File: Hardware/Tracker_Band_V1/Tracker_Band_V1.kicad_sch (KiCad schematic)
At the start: 78 parts, among them J1 USB_C_USB20, Q1 SSM6L56FE, SW1 EVP-AVAA1A, SW2 EVP-AVAA1A, U1 ESP32-C3-MINI-1-N4, U2 BNO085, U3 RT8010, U4 MCP73832-2-AC, U5 LM66200, U6 IN-PI15TAT5R5G5B, U7 IN-PI15TAT5R5G5B, U8 IN-PI15TAT5R5G5B, U9 IN-PI15TAT5R5G5B, X1 32.768kHz

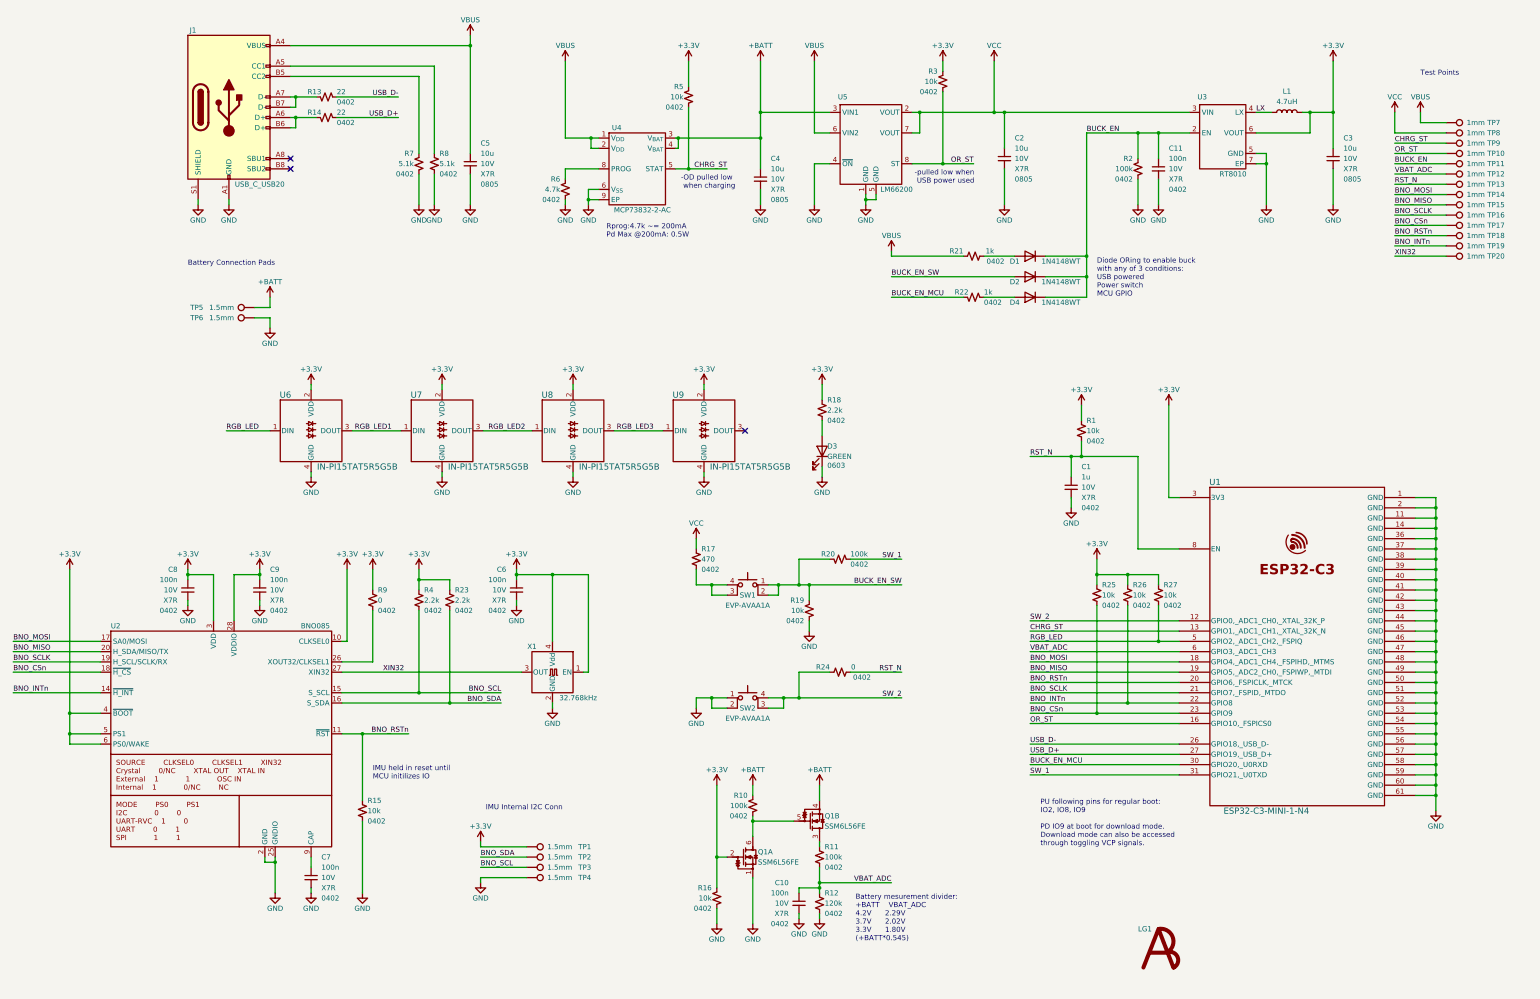
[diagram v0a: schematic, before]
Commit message: SCH & PCB Finalized for review
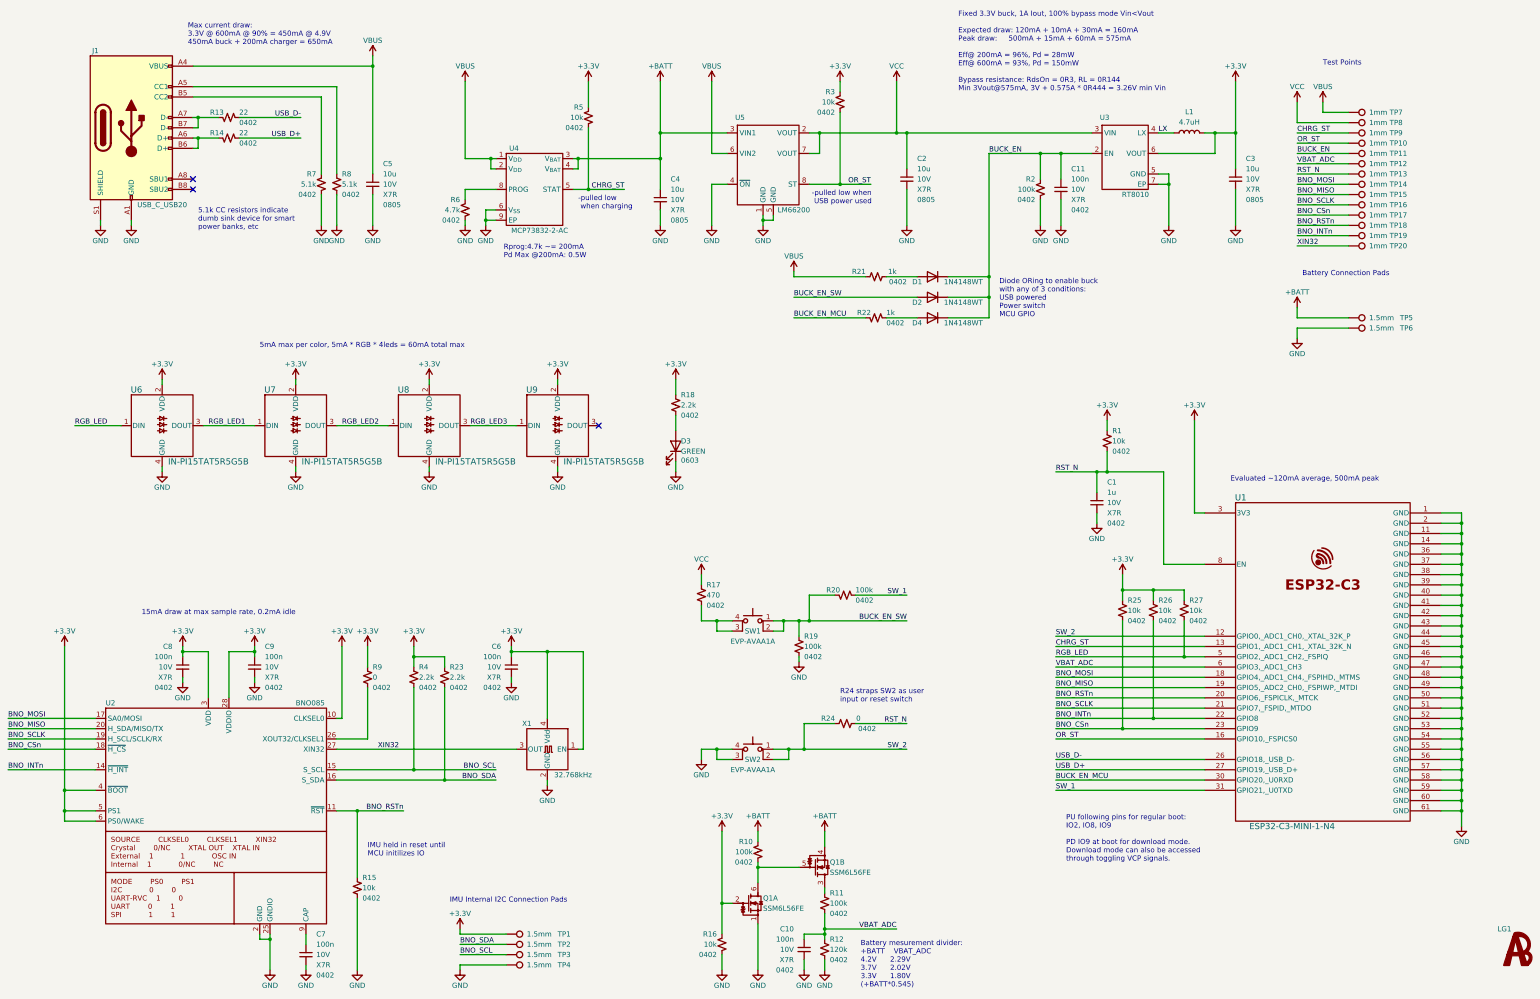
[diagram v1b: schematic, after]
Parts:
- R19: value 10k -> 100k
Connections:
- net GND: now also SW2.3 (K), SW2.4 (A); no longer SW2.1, SW2.2
- net SW_2: now also SW2.1, SW2.2; no longer SW2.3 (K), SW2.4 (A)
- now unconnected: U1.10 (NC), U1.15 (NC), U1.17 (NC), U1.24 (NC), U1.25 (NC), U1.28 (NC), U1.29 (NC), U1.32 (NC), U1.33 (NC), U1.34 (NC), U1.35 (NC), U1.4 (NC), U1.7 (NC), U1.9 (NC), U2.1 (PIN1), U2.12 (PIN12), U2.13 (PIN13), U2.21 (PIN21), U2.22 (PIN22), U2.23 (PIN23), U2.24 (PIN24), U2.7 (PIN7), U2.8 (PIN8)
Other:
- note added: "-pulled low when charging"
- note added: "15mA draw at max sample rate, 0.2mA idle"
- note added: "5.1k CC resistors indicate dumb sink device for smart power banks, etc"
- note added: "5mA max per color, 5mA * RGB * 4leds = 60mA total max"
- note added: "Evaluated ~120mA average, 500mA peak"
- note added: "Fixed 3.3V buck, 1A Iout, 100% bypass mode Vin<Vout Expected draw: 120mA + 10mA + 30mA = 160mA Peak draw: 500mA + 15mA + 60mA = 575mA Eff@ 200mA = 96%, Pd = 28mW Eff@ 600mA = 93%, Pd = 150mW Bypass resistance: RdsOn = 0R3, RL = 0R144 Min 3Vout@575mA, 3V + 0.575A * 0R444 = 3.26V min Vin"
- note added: "IMU Internal I2C Connection Pads"
- note added: "Max current draw: 3.3V @ 600mA @ 90% = 450mA @ 4.9V 450mA buck + 200mA charger = 650mA"
- note added: "R24 straps SW2 as user input or reset switch"
- note removed: "-OD pulled low when charging"
- note removed: "IMU Internal I2C Conn"
- company: (none) -> BCIT BENG 2024
- title: (none) -> SilhouetteSync V1
- moved on the sheet: C1, C10, C11, C2, C3, C4, C5, C6, C7, C8, C9, D1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
